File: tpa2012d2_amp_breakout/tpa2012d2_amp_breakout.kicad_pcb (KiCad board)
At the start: 2 copper layers, 40 x 20 mm, 14 parts, among them J101 Conn_01x07_Female, J102 SPK L, J103 SPK R, J104 AudioJack3, U301 TPA2012D2

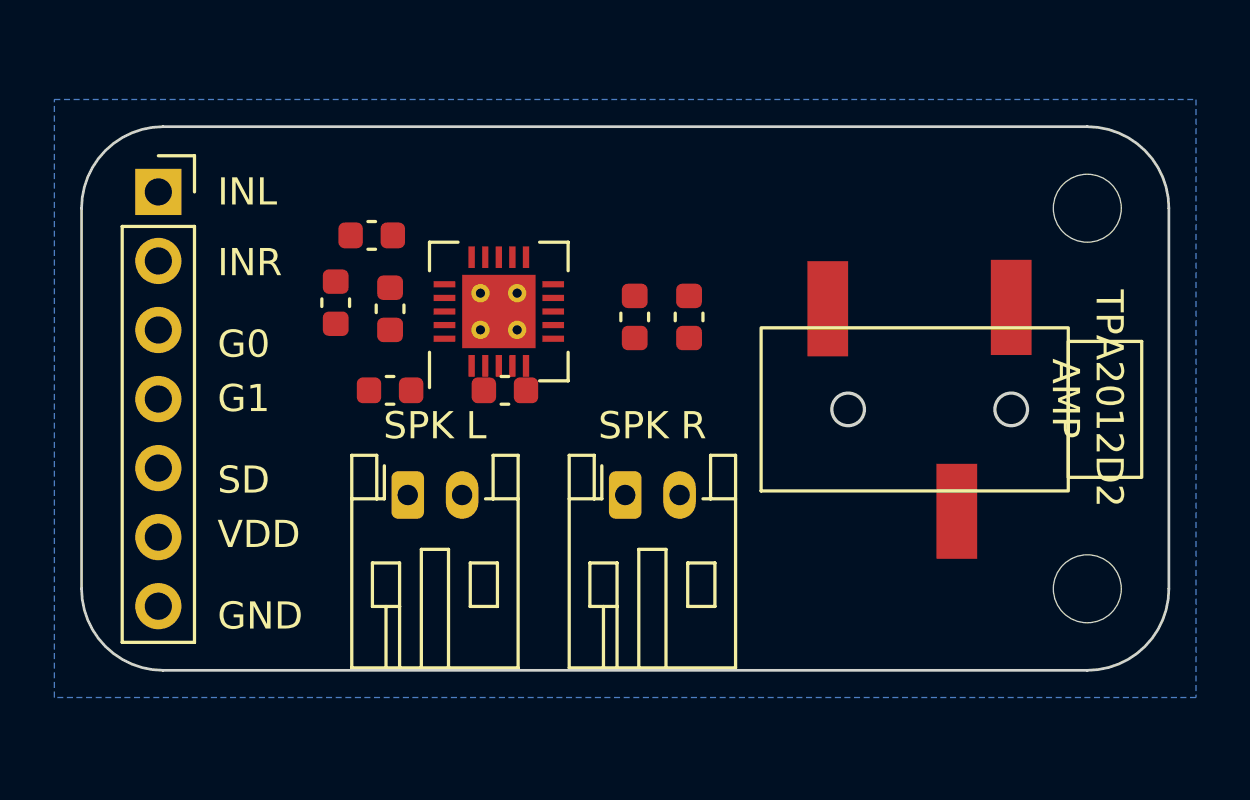
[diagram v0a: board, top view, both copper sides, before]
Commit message: WIP
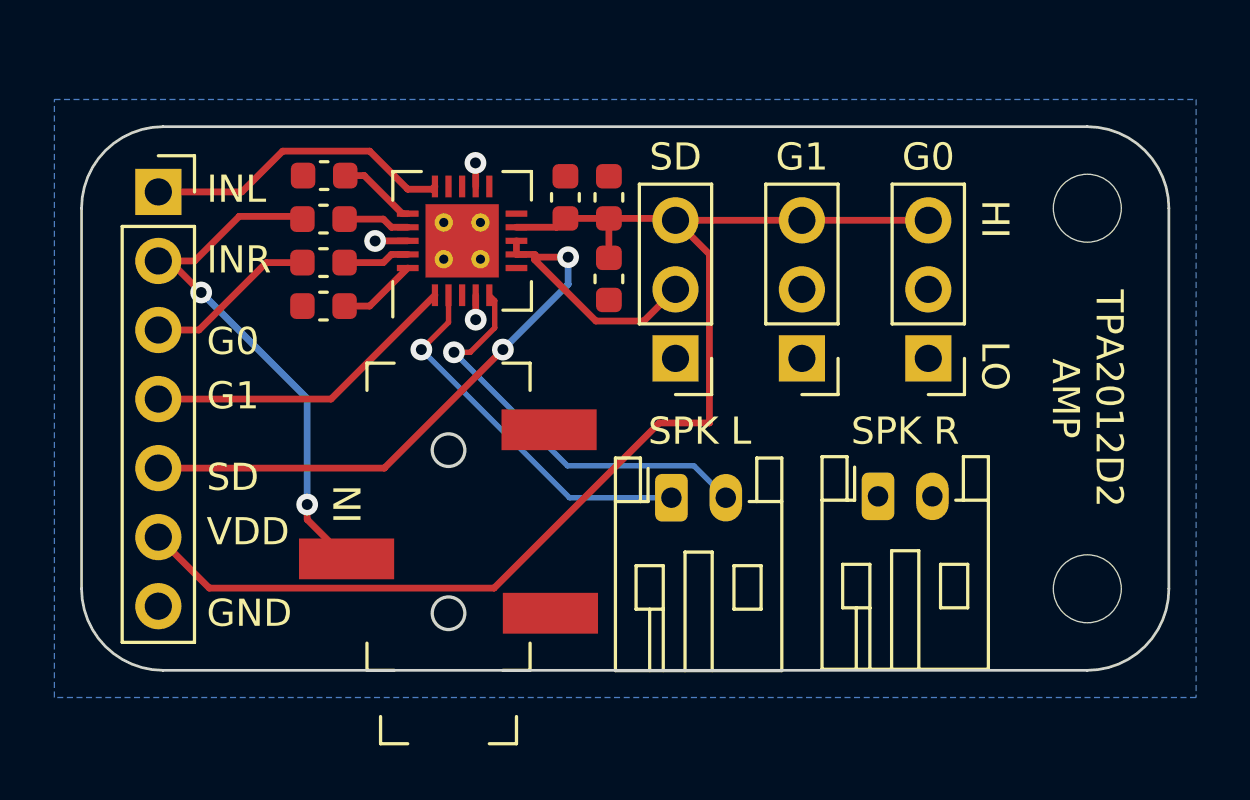
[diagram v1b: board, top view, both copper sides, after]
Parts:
- added J105: SD, Connector_PinHeader_2.54mm:PinHeader_1x03_P2.54mm_Vertical, F.Cu at (161.8, 88.5)
- added J106: G0, Connector_PinHeader_2.54mm:PinHeader_1x03_P2.54mm_Vertical, F.Cu at (171.2, 88.5)
- added J107: G1, Connector_PinHeader_2.54mm:PinHeader_1x03_P2.54mm_Vertical, F.Cu at (166.5, 88.5)
- moved J104 24.7 mm to (153.5, 100.0), turned to 0 degrees
- moved J102 9.70 mm to (161.7, 93.7)
- moved J103 9.30 mm to (169.3, 93.6)
- moved C305 5.61 mm to (159.4, 85.6), turned to 90 degrees
- moved C301 5.30 mm to (159.4, 82.6)
- moved C307 5.09 mm to (157.8, 82.6)
- moved C302 3.95 mm to (148.9, 86.6)
- moved C304 3.11 mm to (148.9, 83.4), turned to 0 degrees
- moved C303 2.98 mm to (148.9, 85.0), turned to 180 degrees
- moved U301 2.93 mm to (154.0, 84.2)
- moved C306 2.81 mm to (148.9, 81.8), turned to 180 degrees
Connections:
- J101 pad 1: INL- -> G0
- J101 pad 3: G0 -> INL-
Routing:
- net VDD: track 0.00 -> 48.3 mm
- net SD: track 0.00 -> 28.1 mm, vias 0 -> 2
- net INR-: track 0.00 -> 20.1 mm, vias 0 -> 2
- net /TPA2012D2/OUTL-: track 0.00 -> 15.4 mm, vias 0 -> 1
- net /TPA2012D2/OUTL+: track 0.00 -> 13.9 mm, vias 0 -> 1
- net G1: track 0.00 -> 11.8 mm
- net G0: track 0.00 -> 11.4 mm
- net INL-: track 0.00 -> 6.33 mm
- net GND: track 0.00 -> 2.97 mm, vias 0 -> 3
- net Net-(C302-Pad1): track 0.00 -> 2.90 mm
- net Net-(C306-Pad1): track 0.00 -> 2.88 mm
- net Net-(C304-Pad2): track 0.00 -> 2.45 mm
- net Net-(C303-Pad1): track 0.00 -> 2.45 mm
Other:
- board text added: "HI"
- board text added: "IN"
- board text added: "LO"

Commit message: WIP
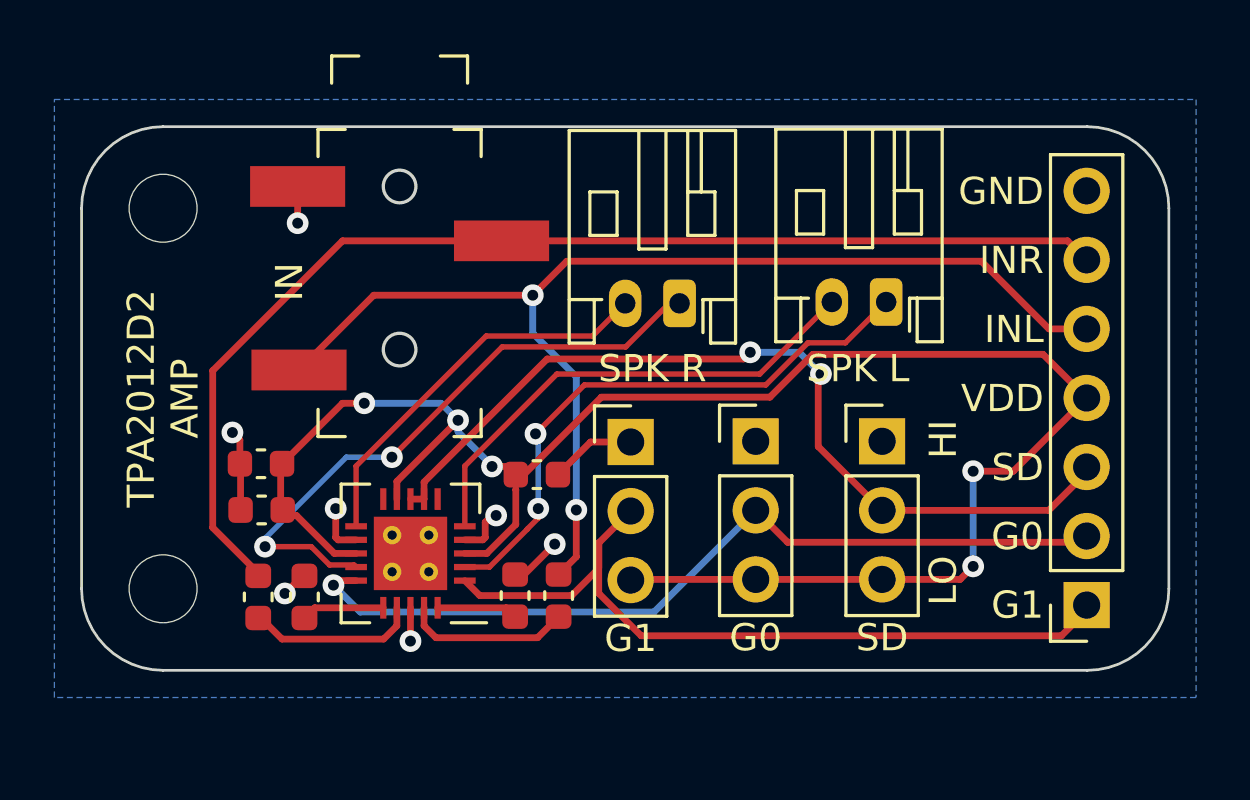
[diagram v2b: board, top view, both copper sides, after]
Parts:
- removed the REF** at (177.0, 97.0)
- removed the REF** at (177.0, 83.0)
- added REF**: MountingHole_2.5mm, MountingHole:MountingHole_2.5mm, F.Cu at (143.0, 97.0)
- added REF**: MountingHole_2.5mm, MountingHole:MountingHole_2.5mm, F.Cu at (143.0, 83.0)
- moved J101 37.4 mm to (177.0, 97.6), turned to 180 degrees
- moved J104 20.0 mm to (151.7, 80.1), turned to 180 degrees
- moved C301 16.1 mm to (146.6, 92.4), turned to 180 degrees
- moved C307 16.0 mm to (146.6, 94.1), turned to 180 degrees
- moved C306 15.5 mm to (148.2, 97.3), turned to 90 degrees
- moved C303 15.0 mm to (157.6, 97.2), turned to 90 degrees
- moved C304 14.1 mm to (146.5, 97.3), turned to -90 degrees
- moved C302 12.8 mm to (155.9, 97.2), turned to 90 degrees
- moved U301 11.7 mm to (152.1, 95.7), turned to 180 degrees
- moved J102 10.7 mm to (169.6, 86.5), turned to 180 degrees
- moved J103 10.2 mm to (162.0, 86.5), turned to 180 degrees
- moved J105 8.19 mm to (169.4, 91.6), turned to 0 degrees
- moved C305 7.67 mm to (156.8, 92.8), turned to 180 degrees
- moved J106 7.04 mm to (164.8, 91.6), turned to 0 degrees
- moved J107 7.01 mm to (160.2, 91.6), turned to 0 degrees
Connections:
- J101 pad 1: G0 -> G1
- J101 pad 2: INR- -> G0
- J101 pad 3: INL- -> SD
- J101 pad 4: G1 -> VDD
- J101 pad 5: SD -> INL-
- J101 pad 6: VDD -> INR-
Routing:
- net INL-: track 6.33 -> 42.9 mm, vias 0 -> 2
- net /TPA2012D2/OUTR+: track 0.00 -> 22.8 mm, vias 0 -> 2
- net INR-: track 20.1 -> 42.7 mm, vias 2 -> 0
- net G0: track 11.4 -> 31.8 mm, vias 0 -> 1
- net VDD: track 48.3 -> 68.4 mm, vias 0 -> 5
- net G1: track 11.8 -> 29.3 mm
- net /TPA2012D2/OUTR-: track 0.00 -> 14.6 mm
- net GND: track 2.97 -> 15.3 mm, vias 3 -> 7
- net /TPA2012D2/OUTL+: track 13.9 -> 21.5 mm, vias 1 -> 2
- net SD: track 28.1 -> 32.4 mm
- net Net-(C304-Pad2): track 2.45 -> 6.19 mm
- net Net-(C303-Pad1): track 2.45 -> 6.12 mm
- net /TPA2012D2/OUTL-: track 15.4 -> 18.2 mm, vias 1 -> 0
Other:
- board text added: "V1"
